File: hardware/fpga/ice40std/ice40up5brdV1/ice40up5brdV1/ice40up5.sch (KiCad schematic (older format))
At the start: 3 parts, among them U1 ICE40UP5K-SG48ITR

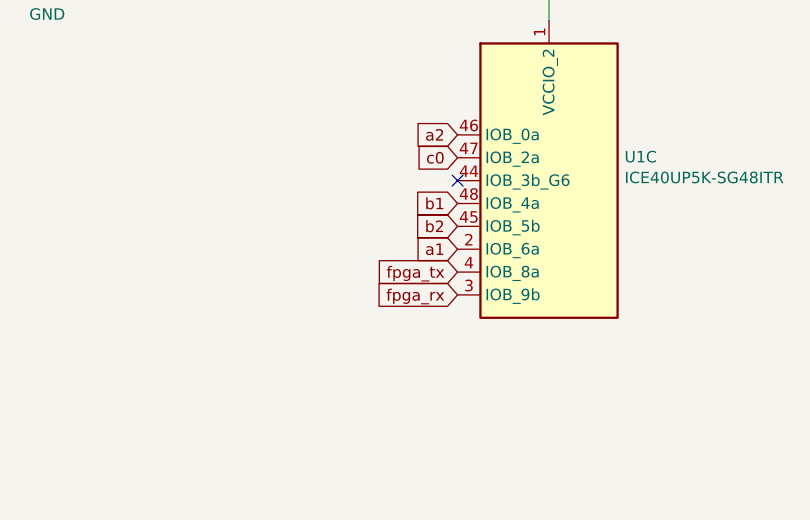
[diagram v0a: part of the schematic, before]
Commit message: FPGA improvements, SPEC changed!
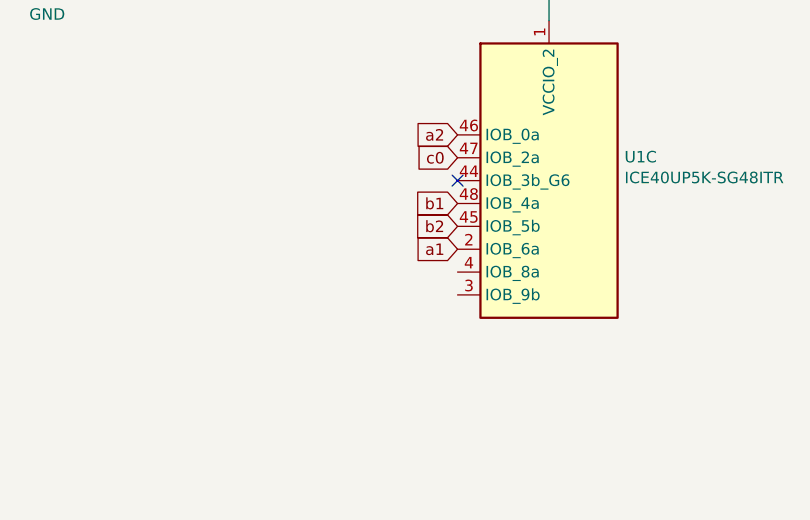
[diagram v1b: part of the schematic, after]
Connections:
- net fpga_rx: no longer names the net of U1.3 (IOB_9b)
- net fpga_tx: no longer names the net of U1.4 (IOB_8a)
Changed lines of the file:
@@
 Wire Wire Line
 	3150 2500 3150 2700
-Text GLabel 7050 3900 0    50   Input ~ 0
-fpga_tx
-Text GLabel 7050 4000 0    50   Input ~ 0
-fpga_rx
 $Comp
 L Device:C C1

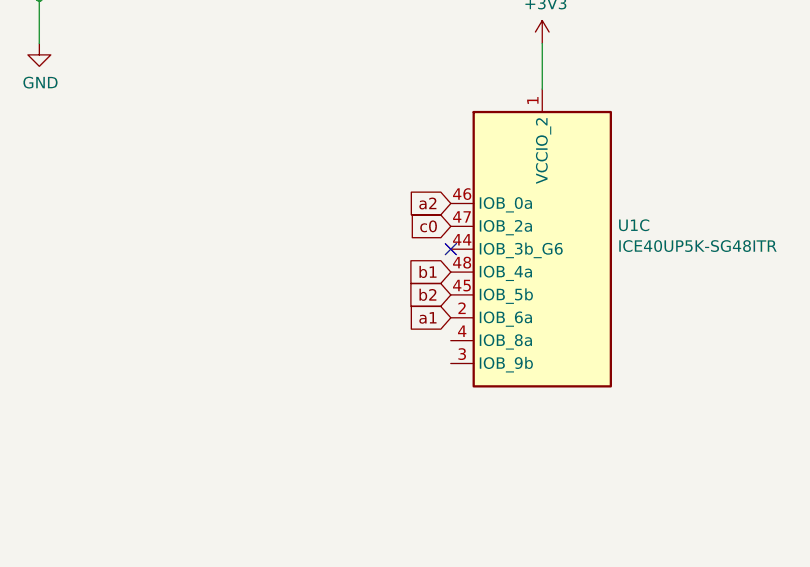
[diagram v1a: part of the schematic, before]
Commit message: FPGA improvements, SPEC changed!
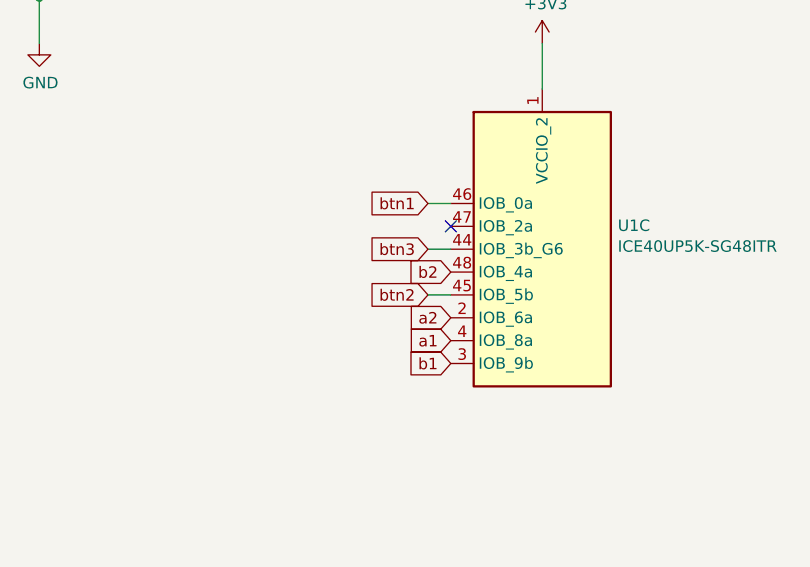
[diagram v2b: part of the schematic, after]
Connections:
- net a1: now also U1.4 (IOB_8a); no longer U1.2 (IOB_6a)
- net a2: now also U1.2 (IOB_6a); no longer U1.46 (IOB_0a)
- net b1: now also U1.3 (IOB_9b); no longer U1.48 (IOB_4a)
- net b2: now also U1.48 (IOB_4a); no longer U1.45 (IOB_5b)
- net btn3: now reaches U1.44 (IOB_3b_G6)
- net c0: no longer names the net of U1.47 (IOB_2a)
- new net btn1: U1.46 (IOB_0a)
- new net btn2: U1.45 (IOB_5b)
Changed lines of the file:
@@
 Text GLabel 2750 4700 0    50   Input ~ 0
 d7
+Text GLabel 7050 3900 0    50   Input ~ 0
+a1
+Text GLabel 7050 4000 0    50   Input ~ 0
+b1
 Text GLabel 7050 3800 0    50   Input ~ 0
-a1
+a2
 Text GLabel 7050 3600 0    50   Input ~ 0
-b1
-Text GLabel 7050 3300 0    50   Input ~ 0
-a2
-Text GLabel 7050 3700 0    50   Input ~ 0
 b2
-Text GLabel 7050 3400 0    50   Input ~ 0
-c0
-NoConn ~ 7050 3500
 $Comp
 L power:+3V3 #PWR01
@@
 Text GLabel 2750 4300 0    50   Input ~ 0
 l3
+Text GLabel 6950 3300 0    50   Input ~ 0
+btn1
+Wire Wire Line
+	6950 3300 7050 3300
+Text GLabel 6950 3700 0    50   Input ~ 0
+btn2
+Wire Wire Line
+	6950 3700 7050 3700
+Text GLabel 6950 3500 0    50   Input ~ 0
+btn3
+Wire Wire Line
+	6950 3500 7050 3500
+NoConn ~ 7050 3400
 $EndSCHEMATC

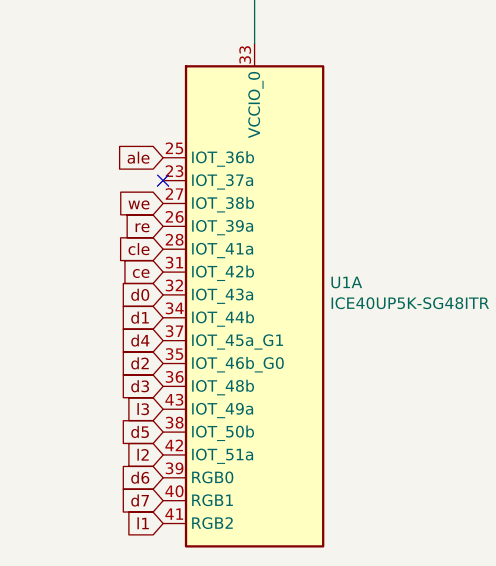
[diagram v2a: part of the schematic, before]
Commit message: ice40qfn restarted: simplest design ready?
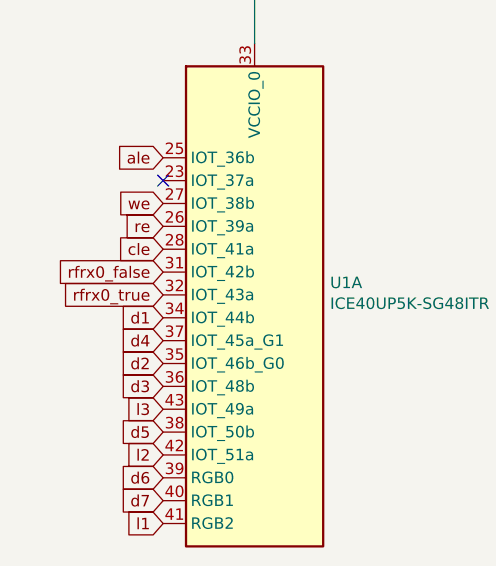
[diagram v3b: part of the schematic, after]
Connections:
- net ce renamed rfrx0_false
- net d0 renamed rfrx0_true
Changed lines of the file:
@@
 cle
 Text GLabel 2750 3700 0    50   Input ~ 0
-ce
+rfrx0_false
 Text GLabel 2750 3800 0    50   Input ~ 0
-d0
+rfrx0_true
 Text GLabel 2750 3900 0    50   Input ~ 0
 d1

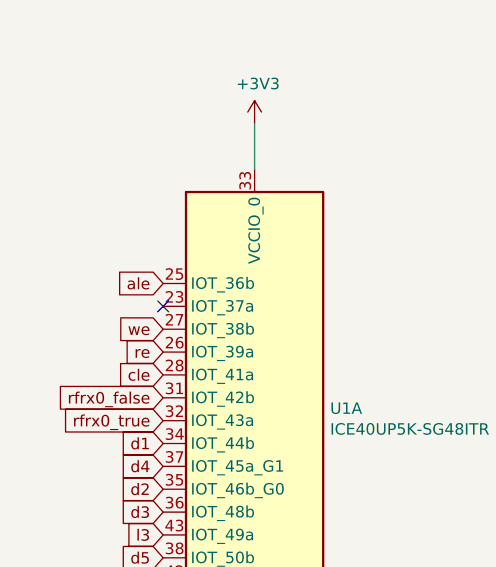
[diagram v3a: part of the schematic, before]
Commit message: ice40qfn restarted: simplest design ready?
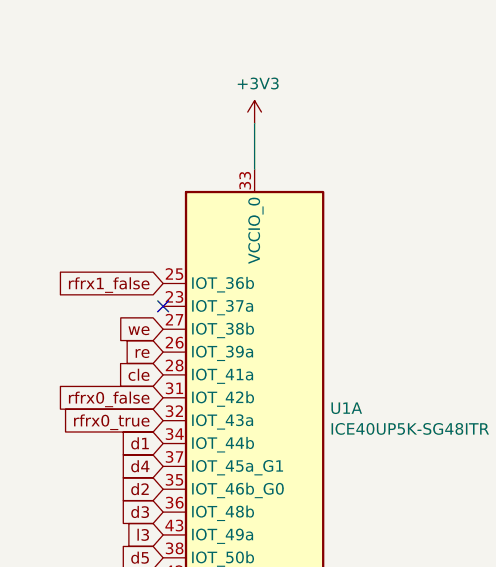
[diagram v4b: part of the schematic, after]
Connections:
- net ale renamed rfrx1_false
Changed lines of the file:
@@
 	1    0    0    -1
 $EndComp
-Text GLabel 2750 3200 0    50   Input ~ 0
-ale
 Text GLabel 2750 3500 0    50   Input ~ 0
 re
@@
 Wire Wire Line
 	5250 2400 5600 2400
-NoConn ~ 2750 3300
 Text GLabel 2750 4800 0    50   Input ~ 0
 l1
@@
 	6950 3500 7050 3500
 NoConn ~ 7050 3400
+Text GLabel 2750 3200 0    50   Input ~ 0
+rfrx1_false
+NoConn ~ 2750 3300
 $EndSCHEMATC

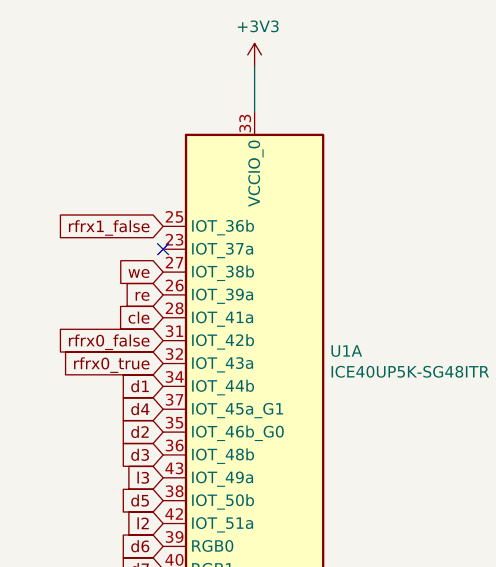
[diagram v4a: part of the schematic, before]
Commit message: ice40qfn restarted: simplest design ready?
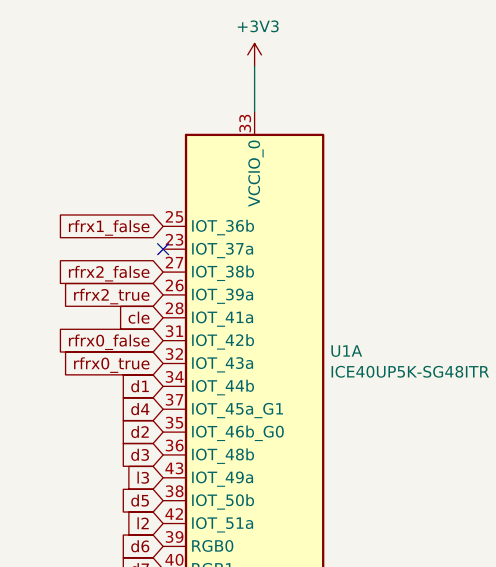
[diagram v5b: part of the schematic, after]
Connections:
- net re renamed rfrx2_true
- net we renamed rfrx2_false
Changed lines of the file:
@@
 $EndComp
 Text GLabel 2750 3500 0    50   Input ~ 0
-re
+rfrx2_true
 Text GLabel 2750 3400 0    50   Input ~ 0
-we
+rfrx2_false
 Text GLabel 2750 3600 0    50   Input ~ 0
 cle

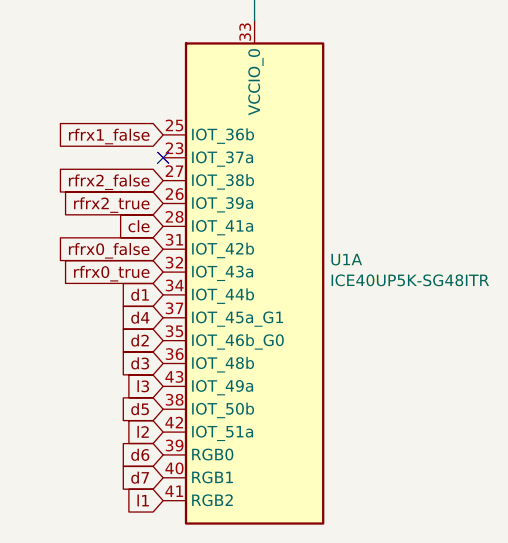
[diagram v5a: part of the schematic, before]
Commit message: ice40qfn restarted: simplest design ready?
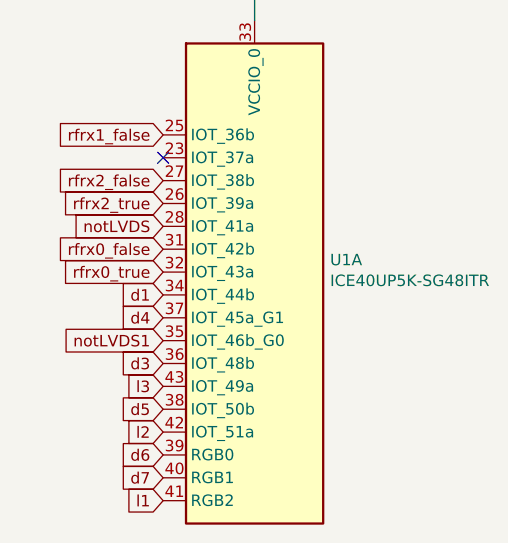
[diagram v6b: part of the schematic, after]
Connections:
- net cle renamed notLVDS
- net d2 renamed notLVDS1
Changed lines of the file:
@@
 rfrx2_false
 Text GLabel 2750 3600 0    50   Input ~ 0
-cle
+notLVDS
 Text GLabel 2750 3700 0    50   Input ~ 0
 rfrx0_false
@@
 d1
 Text GLabel 2750 4100 0    50   Input ~ 0
-d2
+notLVDS1
 Text GLabel 2750 4200 0    50   Input ~ 0
 d3

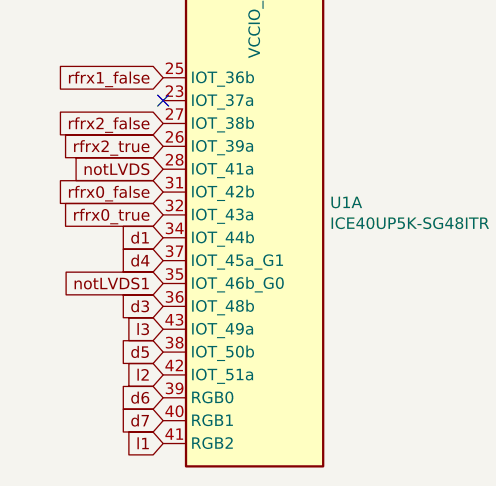
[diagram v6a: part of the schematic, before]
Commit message: ice40qfn restarted: simplest design ready?
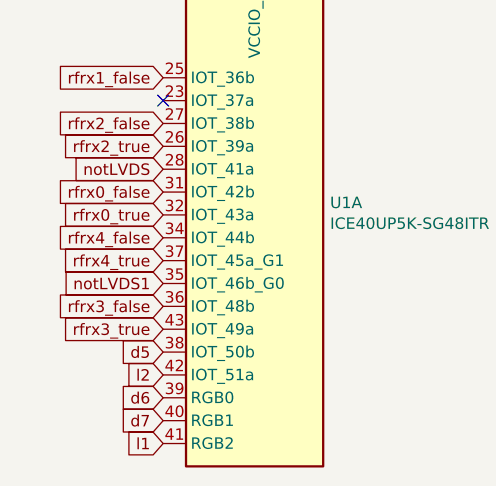
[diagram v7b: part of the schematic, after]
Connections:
- net d1 renamed rfrx4_false
- net d3 renamed rfrx3_false
- net d4 renamed rfrx4_true
- net l3 renamed rfrx3_true
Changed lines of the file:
@@
 rfrx0_true
 Text GLabel 2750 3900 0    50   Input ~ 0
-d1
+rfrx4_false
 Text GLabel 2750 4100 0    50   Input ~ 0
 notLVDS1
 Text GLabel 2750 4200 0    50   Input ~ 0
-d3
+rfrx3_false
 Text GLabel 2750 4000 0    50   Input ~ 0
-d4
+rfrx4_true
 Text GLabel 2750 4400 0    50   Input ~ 0
 d5
@@
 l2
 Text GLabel 2750 4300 0    50   Input ~ 0
-l3
+rfrx3_true
 Text GLabel 6950 3300 0    50   Input ~ 0
 btn1

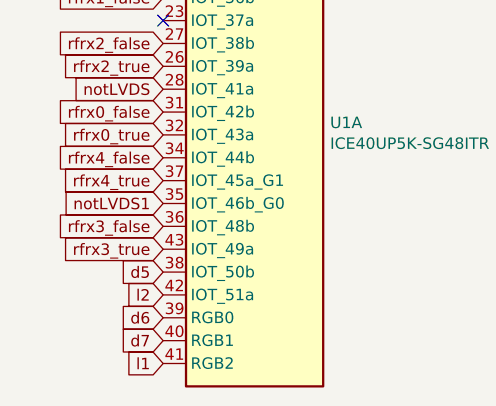
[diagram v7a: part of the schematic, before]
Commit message: ice40qfn restarted: simplest design ready?
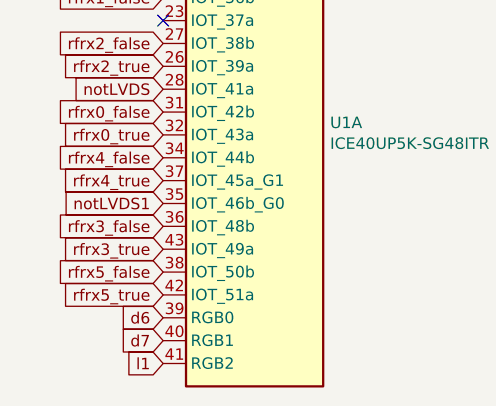
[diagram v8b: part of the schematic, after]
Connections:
- net d5 renamed rfrx5_false
- net l2 renamed rfrx5_true
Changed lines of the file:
@@
 rfrx4_true
 Text GLabel 2750 4400 0    50   Input ~ 0
-d5
+rfrx5_false
 Text GLabel 2750 4600 0    50   Input ~ 0
 d6
@@
 l1
 Text GLabel 2750 4500 0    50   Input ~ 0
-l2
+rfrx5_true
 Text GLabel 2750 4300 0    50   Input ~ 0
 rfrx3_true
